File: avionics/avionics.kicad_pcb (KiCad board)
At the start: 4 copper layers, 103 x 60 mm, 68 parts, among them J1 BAT Balancing leads, J2 BAT, J3 PYRO_0, J4 Servo_0, J5 Servo_1, J6 Servo_2, J7 Servo_3, Q1 AO3400A, Q2 AO3401A, U1 Teensy4.1, U2 BMI088, U3 BMP280, U4 MMC5983MA, U5 TPS548B23VANR, U6 74AHCT125

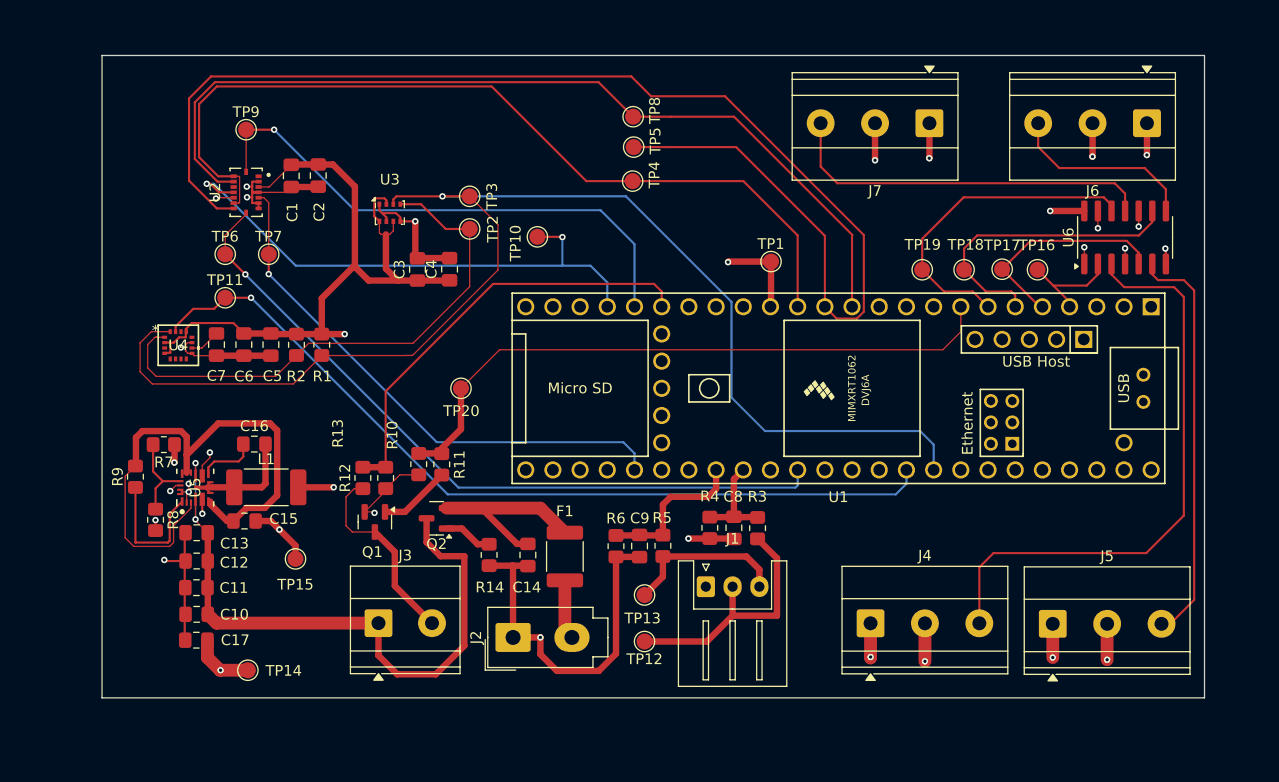
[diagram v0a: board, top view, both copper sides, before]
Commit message: hw: make board smaller, misc hotfixes
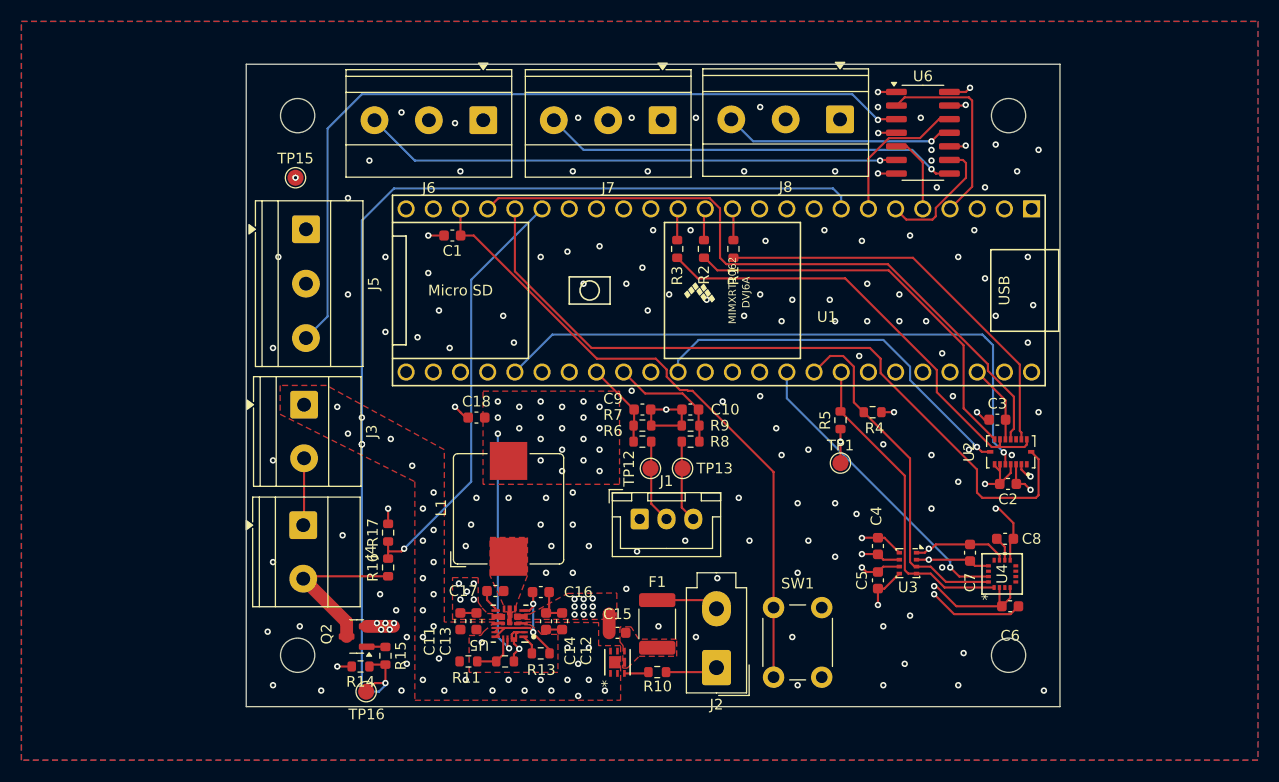
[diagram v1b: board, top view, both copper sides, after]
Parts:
- removed the Q2 at (118.8, 86.4)
- removed TP10: TP_INT_GYR, TestPoint:TestPoint_Pad_D1.5mm
- removed TP11: TP_MAG_INT, TestPoint:TestPoint_Pad_D1.5mm
- removed TP14: TP_5V, TestPoint:TestPoint_Pad_D1.5mm
- removed the TP16 at (174.9, 63.2)
- removed TP17: TP_SERVO_1, TestPoint:TestPoint_Pad_D1.5mm
- removed TP18: TP_SERVO_2, TestPoint:TestPoint_Pad_D1.5mm
- removed TP19: TP_SERVO_3, TestPoint:TestPoint_Pad_D1.5mm
- removed TP2: TP_I2C_SCL, TestPoint:TestPoint_Pad_D1.5mm
- removed TP3: TP_I2C_SDA, TestPoint:TestPoint_Pad_D1.5mm
- removed TP4: TP_MISO, TestPoint:TestPoint_Pad_D1.5mm
- removed TP5: TP_MOSI, TestPoint:TestPoint_Pad_D1.5mm
- removed TP6: TP_SCK, TestPoint:TestPoint_Pad_D1.5mm
- removed TP7: TP_CS_GYR, TestPoint:TestPoint_Pad_D1.5mm
- removed TP8: TP_CS_ACC, TestPoint:TestPoint_Pad_D1.5mm
- removed TP9: TP_INT_ACC, TestPoint:TestPoint_Pad_D1.5mm
- added C1: 100n, Capacitor_SMD:C_0603_1608Metric, F.Cu at (120.2, 60.0)
- added J3: SW_ARM, TerminalBlock_Phoenix:TerminalBlock_Phoenix_MKDS-1,5-2_1x02_P5.00mm_Horizontal, F.Cu at (106.4, 75.8)
- added Q1: RF4C050AP, libraries:TRANS_RF4C_ROM, F.Cu at (135.7, 99.9)
- added R1: 33, Resistor_SMD:R_0603_1608Metric, F.Cu at (146.5, 61.2)
- added R2: 33, Resistor_SMD:R_0603_1608Metric, F.Cu at (143.8, 61.2)
- added R3: 33, Resistor_SMD:R_0603_1608Metric, F.Cu at (141.2, 61.2)
- added SW1: ~{SW_GUIDANCE_EN}, Button_Switch_THT:SW_PUSH_6mm, F.Cu at (150.2, 101.2)
- C10: renamed from C9; footprint Capacitor_SMD:C_0805_2012Metric_Pad1.18x1.45mm_HandSolder -> Capacitor_SMD:C_0603_1608Metric
- C11: renamed from C10; footprint Capacitor_SMD:C_0805_2012Metric_Pad1.18x1.45mm_HandSolder -> Capacitor_SMD:C_0603_1608Metric
- C12: renamed from C11; footprint Capacitor_SMD:C_0805_2012Metric_Pad1.18x1.45mm_HandSolder -> Capacitor_SMD:C_0603_1608Metric
- C13: renamed from C12; footprint Capacitor_SMD:C_0805_2012Metric_Pad1.18x1.45mm_HandSolder -> Capacitor_SMD:C_0603_1608Metric
- C14: renamed from C13; footprint Capacitor_SMD:C_0805_2012Metric_Pad1.18x1.45mm_HandSolder -> Capacitor_SMD:C_0603_1608Metric
- C15: renamed from C14; footprint Capacitor_SMD:C_0805_2012Metric_Pad1.18x1.45mm_HandSolder -> Capacitor_SMD:C_0603_1608Metric
- C16: renamed from C15; footprint Capacitor_SMD:C_0805_2012Metric_Pad1.18x1.45mm_HandSolder -> Capacitor_SMD:C_0603_1608Metric
- C17: renamed from C16; footprint Capacitor_SMD:C_0805_2012Metric_Pad1.18x1.45mm_HandSolder -> Capacitor_SMD:C_0603_1608Metric
- C18: renamed from C17; footprint Capacitor_SMD:C_0805_2012Metric_Pad1.18x1.45mm_HandSolder -> Capacitor_SMD:C_0603_1608Metric
- C2: renamed from C1; footprint Capacitor_SMD:C_0805_2012Metric_Pad1.18x1.45mm_HandSolder -> Capacitor_SMD:C_0603_1608Metric
- C3: renamed from C2; footprint Capacitor_SMD:C_0805_2012Metric_Pad1.18x1.45mm_HandSolder -> Capacitor_SMD:C_0603_1608Metric
- C4: renamed from C3; footprint Capacitor_SMD:C_0805_2012Metric_Pad1.18x1.45mm_HandSolder -> Capacitor_SMD:C_0603_1608Metric
- C5: renamed from C4; footprint Capacitor_SMD:C_0805_2012Metric_Pad1.18x1.45mm_HandSolder -> Capacitor_SMD:C_0603_1608Metric
- C6: renamed from C5; footprint Capacitor_SMD:C_0805_2012Metric_Pad1.18x1.45mm_HandSolder -> Capacitor_SMD:C_0603_1608Metric
- C7: renamed from C6; footprint Capacitor_SMD:C_0805_2012Metric_Pad1.18x1.45mm_HandSolder -> Capacitor_SMD:C_0603_1608Metric
- C8: renamed from C7; footprint Capacitor_SMD:C_0805_2012Metric_Pad1.18x1.45mm_HandSolder -> Capacitor_SMD:C_0603_1608Metric
- C9: renamed from C8; footprint Capacitor_SMD:C_0805_2012Metric_Pad1.18x1.45mm_HandSolder -> Capacitor_SMD:C_0603_1608Metric
- F1: value Littelfuse 1812L090 -> Littelfuse 2920L400
- J1: footprint Connector_JST:JST_XH_S3B-XH-A_1x03_P2.50mm_Horizontal -> Connector_JST:JST_XH_B3B-XH-A_1x03_P2.50mm_Vertical
- L1: value 300n -> 300n (SRP1038A-R33M); footprint Inductor_SMD:L_2512_6332Metric_Pad1.52x3.35mm_HandSolder -> Inductor_SMD:L_Bourns_SRP1038C_10.0x10.0mm
- R10: renamed from R14; footprint Resistor_SMD:R_0805_2012Metric_Pad1.20x1.40mm_HandSolder -> Resistor_SMD:R_0603_1608Metric
- R11: renamed from R7; footprint Resistor_SMD:R_0805_2012Metric_Pad1.20x1.40mm_HandSolder -> Resistor_SMD:R_0603_1608Metric
- R12: renamed from R8; footprint Resistor_SMD:R_0805_2012Metric_Pad1.20x1.40mm_HandSolder -> Resistor_SMD:R_0603_1608Metric
- R13: renamed from R9; footprint Resistor_SMD:R_0805_2012Metric_Pad1.20x1.40mm_HandSolder -> Resistor_SMD:R_0603_1608Metric
- R14: renamed from R10; footprint Resistor_SMD:R_0805_2012Metric_Pad1.20x1.40mm_HandSolder -> Resistor_SMD:R_0603_1608Metric
- R15: renamed from R11; footprint Resistor_SMD:R_0805_2012Metric_Pad1.20x1.40mm_HandSolder -> Resistor_SMD:R_0603_1608Metric
- R16: renamed from R12; footprint Resistor_SMD:R_0805_2012Metric_Pad1.20x1.40mm_HandSolder -> Resistor_SMD:R_0603_1608Metric
- R17: renamed from R13; footprint Resistor_SMD:R_0805_2012Metric_Pad1.20x1.40mm_HandSolder -> Resistor_SMD:R_0603_1608Metric
- R4: renamed from R1; footprint Resistor_SMD:R_0805_2012Metric_Pad1.20x1.40mm_HandSolder -> Resistor_SMD:R_0603_1608Metric
- R5: renamed from R2; footprint Resistor_SMD:R_0805_2012Metric_Pad1.20x1.40mm_HandSolder -> Resistor_SMD:R_0603_1608Metric
- R6: renamed from R3; footprint Resistor_SMD:R_0805_2012Metric_Pad1.20x1.40mm_HandSolder -> Resistor_SMD:R_0603_1608Metric
- R7: renamed from R4; footprint Resistor_SMD:R_0805_2012Metric_Pad1.20x1.40mm_HandSolder -> Resistor_SMD:R_0603_1608Metric
- R8: renamed from R5; footprint Resistor_SMD:R_0805_2012Metric_Pad1.20x1.40mm_HandSolder -> Resistor_SMD:R_0603_1608Metric
- R9: renamed from R6; footprint Resistor_SMD:R_0805_2012Metric_Pad1.20x1.40mm_HandSolder -> Resistor_SMD:R_0603_1608Metric
- U2: footprint BMI088:PQFN50P450X300X100-16N -> libraries:PQFN50P450X300X100-16N
- moved U4 79.9 mm to (171.6, 91.6), turned to 90 degrees
- moved C8 75.9 mm to (171.9, 88.3), turned to 180 degrees
- moved U2 75.4 mm to (172.4, 80.2), turned to 180 degrees
- moved C6 73.2 mm to (172.3, 94.6), turned to 0 degrees
- moved C2 72.9 mm to (172.2, 83.2), turned to 180 degrees
- moved J6 71.0 mm to (123.1, 49.2), turned to 180 degrees
- moved C7 70.6 mm to (168.6, 89.6), turned to 90 degrees
- moved C3 67.4 mm to (171.2, 77.2), turned to 180 degrees
- moved J5 64.3 mm to (106.6, 59.4), turned to -90 degrees
- moved U3 58.4 mm to (162.8, 90.6), turned to -90 degrees
- moved R4 51.8 mm to (159.5, 76.5), turned to 180 degrees
- moved R5 51.3 mm to (156.5, 77.2), turned to 90 degrees
- moved C4 50.2 mm to (160.0, 89.0), turned to -90 degrees
- moved C5 49.4 mm to (160.0, 92.2), turned to -90 degrees
- moved J7 45.2 mm to (139.9, 49.2)
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- renumbered J3 to J4, J4 to J5, J5 to J6, J6 to J7, J7 to J8, Q1 to Q2, TP20 to TP16
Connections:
- J4 pad 1: +BATT -> Net-(J3-Pin_2)
- U1 pad 12: /IMU/CS_ACC -> Net-(U1-10_CS_MQSR)
- U1 pad 13: /IMU/MOSI -> Net-(U1-11_MOSI_CTX1)
- U1 pad 14: /IMU/MISO -> Net-(U1-12_MISO_MQSL)
- U1 pad 22: unconnected-(U1-30_CRX3-Pad22) -> Net-(U1-30_CRX3)
- U1 pad 32: /PSU/BAT_CELL_1 -> /PSU/BAT_CELL_0
- U1 pad 33: /PSU/BAT_CELL_0 -> /PSU/BAT_CELL_1
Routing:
- net +5V: track 127.3 -> 24.0 mm, vias 8 -> 23
- net /Barometer/SDA: track 123.0 -> 33.3 mm, vias 1 -> 0
- net /IMU/MOSI: track 122.4 -> 37.6 mm
- net +BATT: track 65.2 -> 1.50 mm, vias 3 -> 29
- net Net-(U1-30_CRX3): track 0.00 -> 60.4 mm
- net /Magnetometer/INT: track 79.2 -> 28.5 mm
- net /IMU/CS_ACC: track 84.6 -> 37.9 mm
- net GND: track 125.8 -> 82.9 mm, vias 23 -> 171
- net Net-(U5-CFG1): track 52.8 -> 13.3 mm, vias 0 -> 2
- net /Pyro_and_servos/PYRO_0: track 60.2 -> 99.2 mm, vias 0 -> 4
- net /IMU/MISO: track 81.5 -> 42.6 mm
- net +3.3V: track 77.9 -> 41.5 mm, vias 3 -> 7
- net SPI_SCK: track 68.7 -> 36.1 mm
- net Net-(J7-Pin_3): track 17.8 -> 39.0 mm, vias 0 -> 1
- net Net-(C15-Pad1): track 21.0 -> 0.00 mm
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- added copper zone on F.Cu, net +5V
- added copper zone on F.Cu, net +BATT
- added copper zone on In2.Cu, net +BATT
- added copper zone on B.Cu, net GND
- added copper zone on F.Cu, net GND
- added copper zone on F.Cu, net Net-(C15-Pad1)
- added copper zone on F.Cu, net Net-(C17-Pad2)
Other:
- board size 103 x 60 mm -> 76 x 60 mm
